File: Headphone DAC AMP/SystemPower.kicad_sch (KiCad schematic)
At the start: 34 parts, among them U1 NCV8187AMTW090TAG, U11 ADP5071AREZ-R7, U6 MCP1727-1802xSN, U7 MCP1727-3302xSN

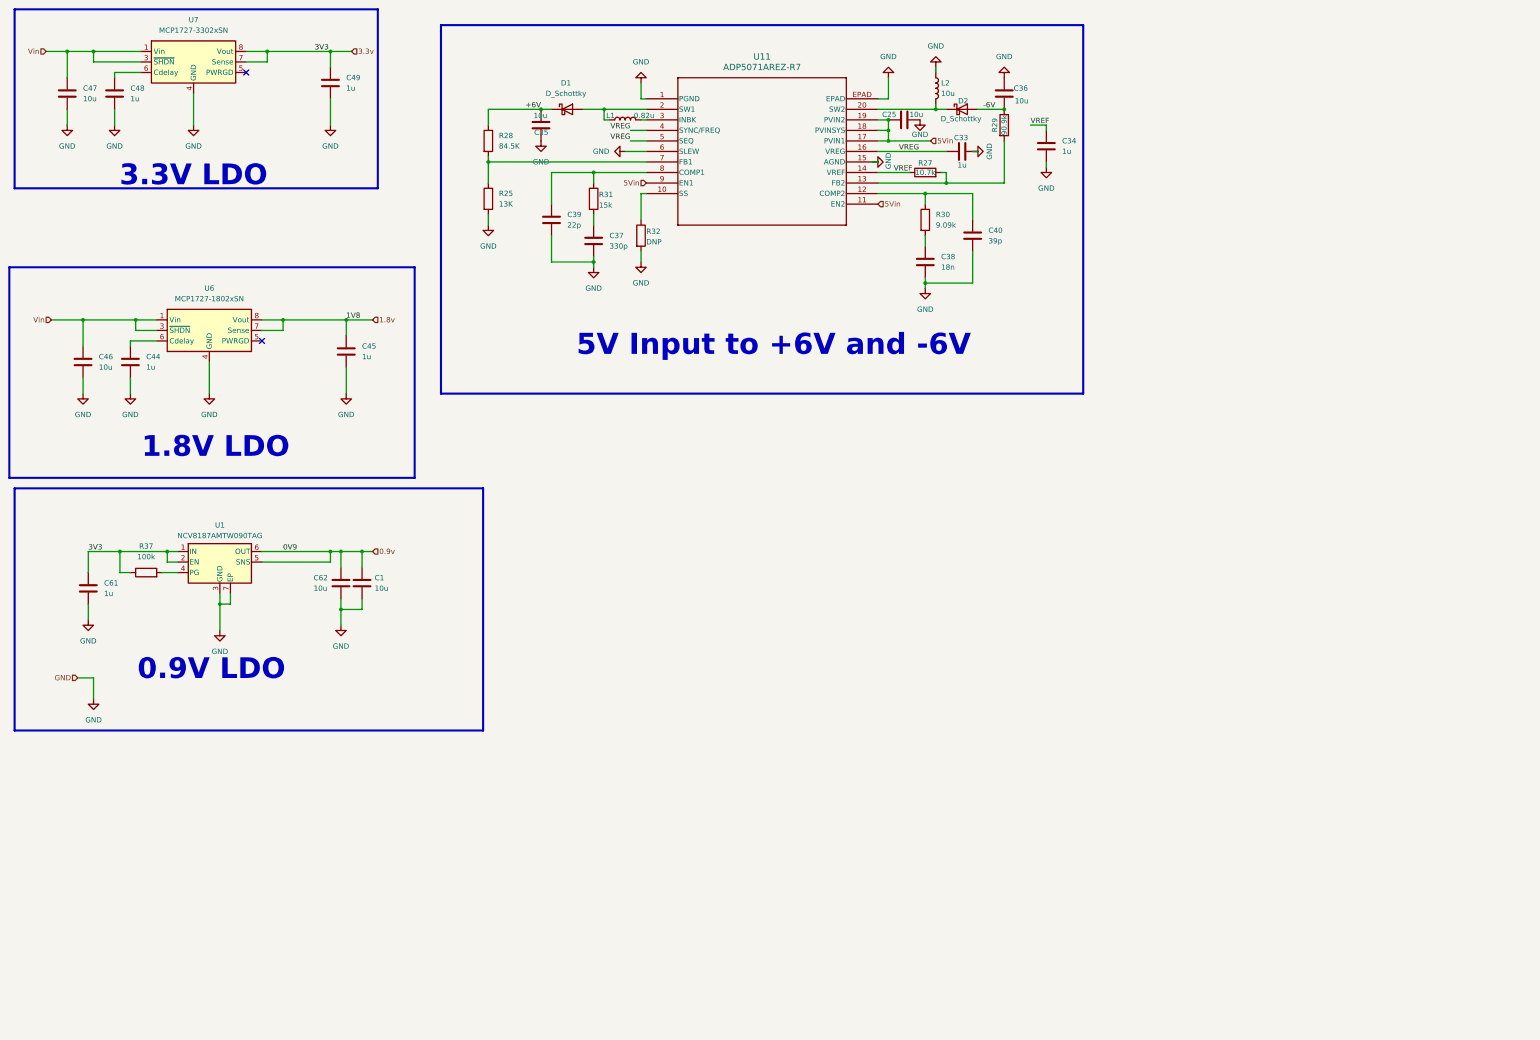
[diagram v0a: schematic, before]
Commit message: Worked on layout briefley
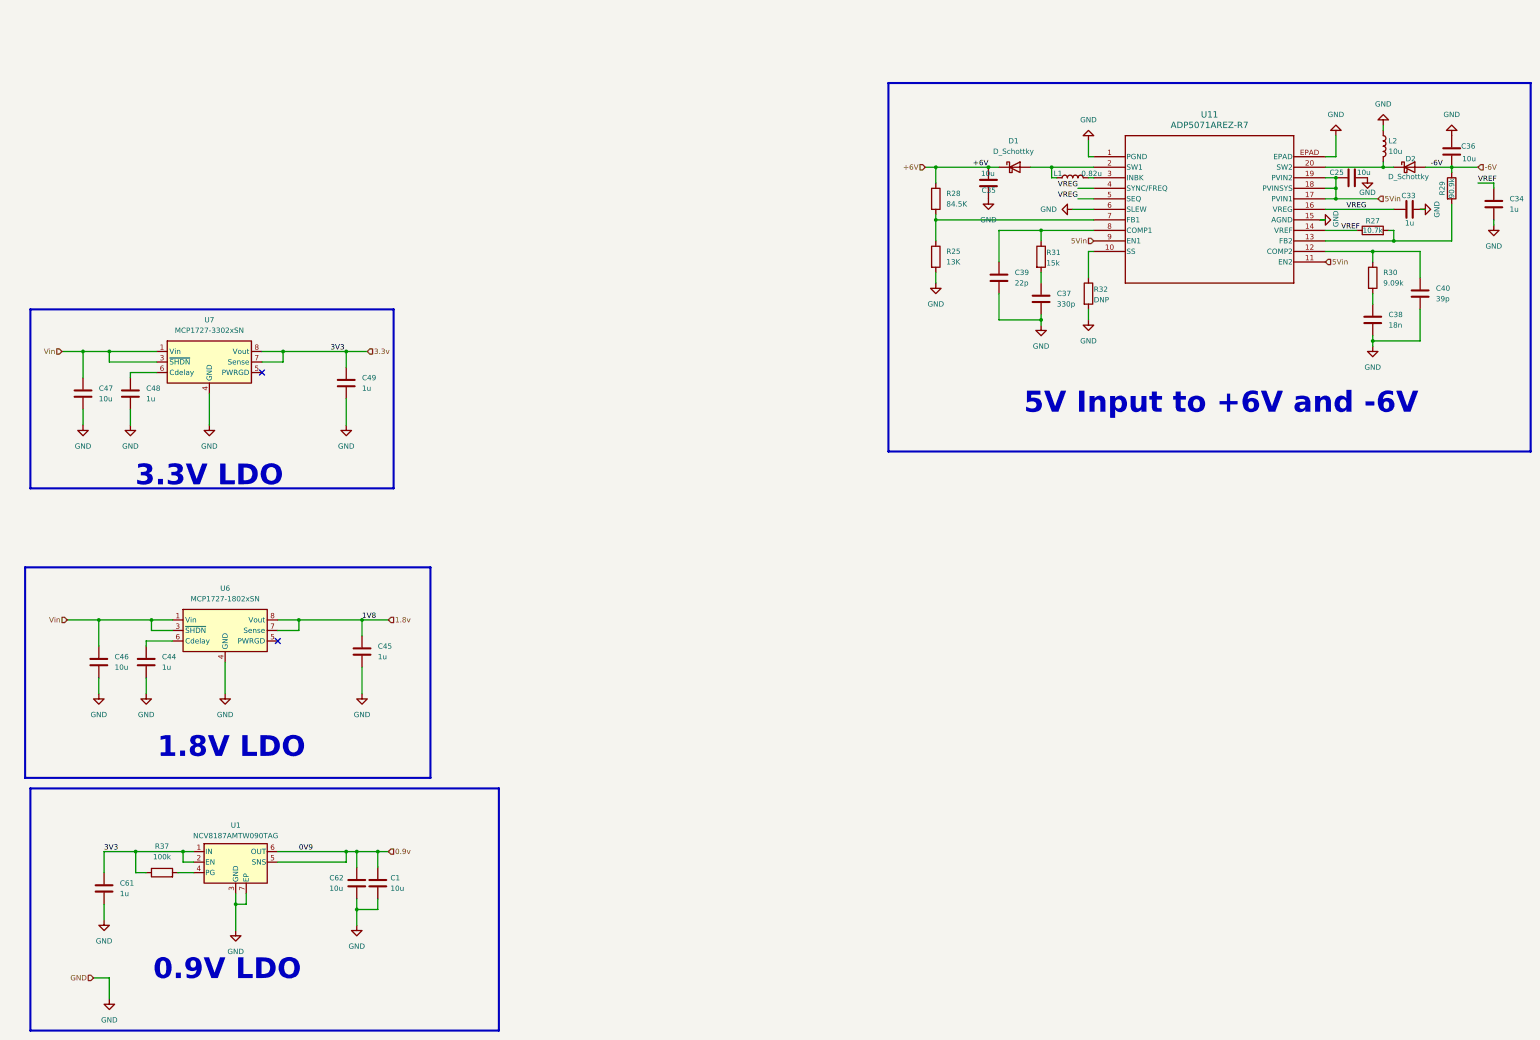
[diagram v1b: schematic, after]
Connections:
- net 3.3v: no longer U1.6 (OUT)
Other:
- moved on the sheet: C1, C25, C33, C34, C35, C36, C37, C38, C39, C40, C44, C45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
